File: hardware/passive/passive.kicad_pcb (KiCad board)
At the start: 2 copper layers, 45 x 17 mm, 8 parts, among them J1 i/O, J2 Conn 1, J3 Conn 2

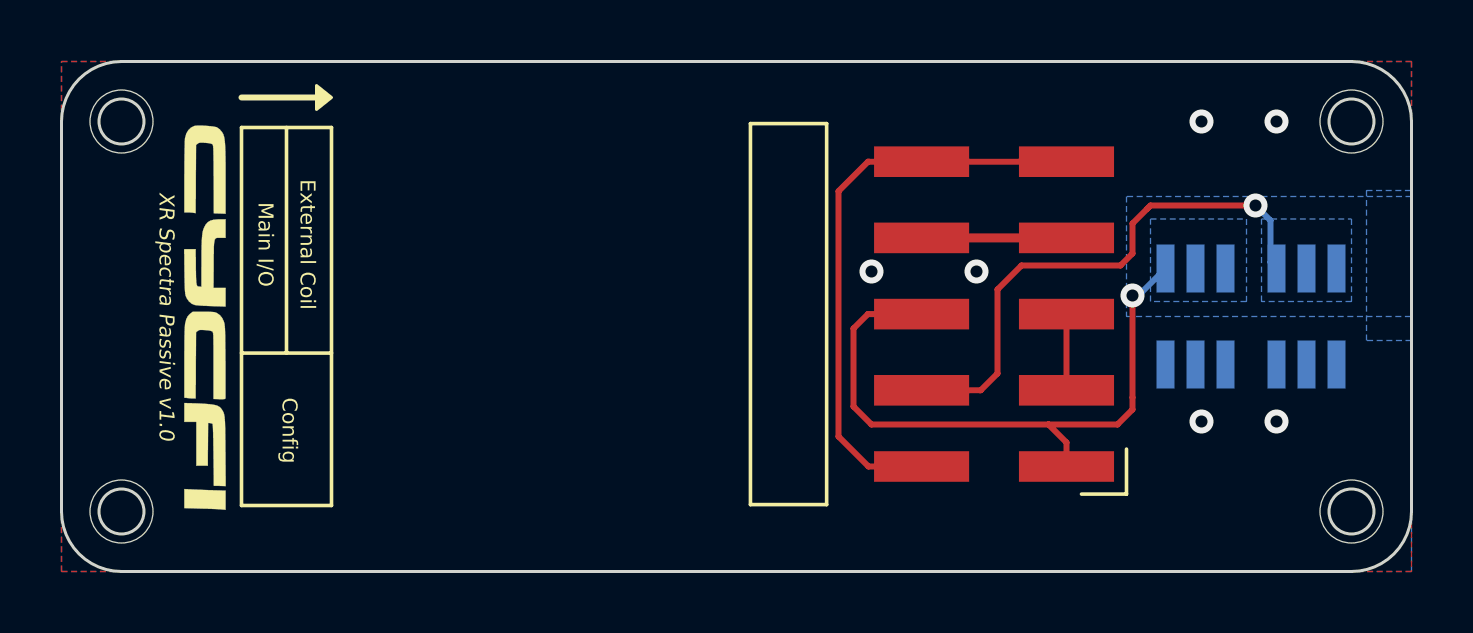
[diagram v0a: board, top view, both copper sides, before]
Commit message: Passive board updates
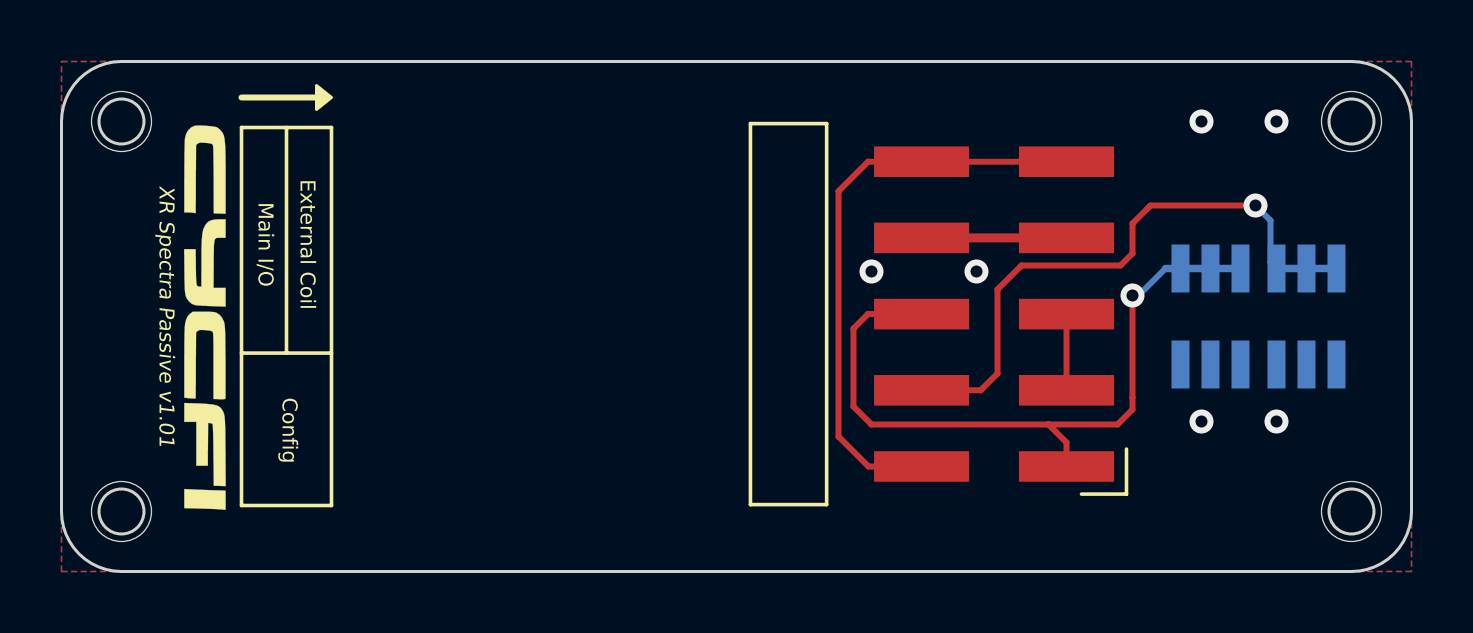
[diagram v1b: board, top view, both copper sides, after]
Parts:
- H1, H2, H3, H4: footprint cycfi_library:mounting_hole_2.1mm -> cycfi_library:mounting_hole_st1.9; moved to F.Cu
- moved J3 0.50 mm to (143.3, 108.5)
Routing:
- net out-: track 21.7 -> 24.2 mm
- net int_coil+: track 18.3 -> 20.3 mm
- removed copper zone on B.Cu, net int_coil+
- removed copper zone on B.Cu, net out-
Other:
- board text added: "XR Spectra Passive v1.01"
- board text removed: "XR Spectra Passive v1.0"
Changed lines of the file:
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@@
     (thickness 1.6)
     (drawings 24)
-    (tracks 42)
+    (tracks 47)
     (zones 0)
     (modules 8)
@@
     (44 Edge.Cuts user)
     (45 Margin user)
-    (46 B.CrtYd user hide)
-    (47 F.CrtYd user hide)
-    (48 B.Fab user hide)
-    (49 F.Fab user hide)
+    (46 B.CrtYd user)
+    (47 F.CrtYd user)
+    (48 B.Fab user)
+    (49 F.Fab user)
   )
   (setup
@@
     (add_net out-)
   )
+  (module cycfi_library:mounting_hole_st1.9 (layer F.Cu)
+    (at 148 115)
+    (descr "Mounting Hole 2.1mm, no annular")
+    (tags "mounting hole 2.1mm no annular")
+    (attr virtual)
+    (fp_text reference H4 (at 0 -3.2) (layer F.SilkS) hide
+      (effects (font (size 1 1) (thickness 0.15)))
+    )
+    (fp_text value MountingHole (at 0 3.2) (layer F.Fab) hide
+      (effects (font (size 1 1) (thickness 0.15)))
+    )
+    (fp_text user %R (at 0.3 0) (layer F.Fab)
+      (effects (font (size 1 1) (thickness 0.15)))
+    )
+    (fp_circle (center 0 0) (end 1.75 0) (layer F.CrtYd) (width 0.05))
+    (pad "" np_thru_hole circle (at 0 0) (size 2 2) (drill 2) (layers *.Cu *.Mask))
+  )
+  (module cycfi_library:mounting_hole_st1.9 (layer F.Cu)
+    (at 148 102)
+    (descr "Mounting Hole 2.1mm, no annular")
+    (tags "mounting hole 2.1mm no annular")
+    (attr virtual)
+    (fp_text reference H3 (at 0 -3.2 180) (layer F.SilkS) hide
+      (effects (font (size 1 1) (thickness 0.15)))
+    )
+    (fp_text value MountingHole (at 0 3.2 180) (layer F.Fab) hide
+      (effects (font (size 1 1) (thickness 0.15)))
+    )
+    (fp_text user %R (at 0.3 0 180) (layer F.Fab)
+      (effects (font (size 1 1) (thickness 0.15)))
+    )
+    (fp_circle (center 0 0) (end 1.75 0) (layer F.CrtYd) (width 0.05))
+    (pad "" np_thru_hole circle (at 0 0) (size 2 2) (drill 2) (layers *.Cu *.Mask))
+  )
+  (module cycfi_library:mounting_hole_st1.9 (layer F.Cu)
+    (at 107 115)
+    (descr "Mounting Hole 2.1mm, no annular")
+    (tags "mounting hole 2.1mm no annular")
+    (attr virtual)
+    (fp_text reference H2 (at 0 -3.2) (layer F.SilkS) hide
+      (effects (font (size 1 1) (thickness 0.15)))
+    )
+    (fp_text value MountingHole (at 0 3.2) (layer F.Fab) hide
+      (effects (font (size 1 1) (thickness 0.15)))
+    )
+    (fp_text user %R (at 0.3 0) (layer F.Fab)
+      (effects (font (size 1 1) (thickness 0.15)))
+    )
+    (fp_circle (center 0 0) (end 1.75 0) (layer F.CrtYd) (width 0.05))
+    (pad "" np_thru_hole circle (at 0 0) (size 2 2) (drill 2) (layers *.Cu *.Mask))
+  )
+  (module cycfi_library:mounting_hole_st1.9 (layer F.Cu)
+    (at 107 102)
+    (descr "Mounting Hole 2.1mm, no annular")
+    (tags "mounting hole 2.1mm no annular")
+    (attr virtual)
+    (fp_text reference H1 (at 0 -3.2) (layer F.SilkS) hide
+      (effects (font (size 1 1) (thickness 0.15)))
+    )
+    (fp_text value MountingHole (at 0 3.2) (layer F.Fab) hide
+      (effects (font (size 1 1) (thickness 0.15)))
+    )
+    (fp_text user %R (at 0.3 0) (layer F.Fab)
+      (effects (font (size 1 1) (thickness 0.15)))
+    )
+    (fp_circle (center 0 0) (end 1.75 0) (layer F.CrtYd) (width 0.05))
+    (pad "" np_thru_hole circle (at 0 0) (size 2 2) (drill 2) (layers *.Cu *.Mask))
+  )
   (module cycfi_library:pin_socket_2x3p_1.00mm_smd_vertical (layer B.Cu)
     (at 146.5 108.5 90)
@@
   )
   (module cycfi_library:pin_socket_2x3p_1.00mm_smd_vertical (layer B.Cu)
-    (at 142.8 108.5 90)
+    (at 143.3 108.5 90)
     (descr "surface-mounted straight pin header, 2x03, 1.00mm pitch, double rows")
     (tags "Surface mounted pin header SMD 2x03 1.00mm double row")
@@
       (rotate (xyz 0 0 0))
     )
-  )
-  (module cycfi_library:mounting_hole_2.1mm (layer B.Cu)
-    (at 148 115)
-    (descr "Mounting Hole 2.1mm, no annular")
-    (tags "mounting hole 2.1mm no annular")
-    (attr virtual)
-    (fp_text reference H4 (at 0 3.2) (layer B.SilkS) hide
-      (effects (font (size 1 1) (thickness 0.15)) (justify mirror))
-    )
-    (fp_text value MountingHole (at 0 -3.2) (layer B.Fab)
-      (effects (font (size 1 1) (thickness 0.15)) (justify mirror))
-    )
-    (fp_text user %R (at 0.3 0) (layer B.Fab)
-      (effects (font (size 1 1) (thickness 0.15)) (justify mirror))
-    )
-    (fp_circle (center 0 0) (end 2.35 0) (layer B.CrtYd) (width 0.05))
-    (pad "" np_thru_hole circle (at 0 0) (size 2.1 2.1) (drill 2.1) (layers *.Cu *.Mask))
-  )
-  (module cycfi_library:mounting_hole_2.1mm (layer B.Cu)
-    (at 148 102)
-    (descr "Mounting Hole 2.1mm, no annular")
-    (tags "mounting hole 2.1mm no annular")
-    (attr virtual)
-    (fp_text reference H3 (at 0 3.2) (layer B.SilkS) hide
-      (effects (font (size 1 1) (thickness 0.15)) (justify mirror))
-    )
-    (fp_text value MountingHole (at 0 -3.2) (layer B.Fab)
-      (effects (font (size 1 1) (thickness 0.15)) (justify mirror))
-    )
-    (fp_text user %R (at 0.3 0) (layer B.Fab)
-      (effects (font (size 1 1) (thickness 0.15)) (justify mirror))
-    )
-    (fp_circle (center 0 0) (end 2.35 0) (layer B.CrtYd) (width 0.05))
-    (pad "" np_thru_hole circle (at 0 0) (size 2.1 2.1) (drill 2.1) (layers *.Cu *.Mask))
-  )
-  (module cycfi_library:mounting_hole_2.1mm (layer B.Cu)
-    (at 107 115)
-    (descr "Mounting Hole 2.1mm, no annular")
-    (tags "mounting hole 2.1mm no annular")
-    (attr virtual)
-    (fp_text reference H2 (at 0 3.2) (layer B.SilkS) hide
-      (effects (font (size 1 1) (thickness 0.15)) (justify mirror))
-    )
-    (fp_text value MountingHole (at 0 -3.2) (layer B.Fab)
-      (effects (font (size 1 1) (thickness 0.15)) (justify mirror))
-    )
-    (fp_text user %R (at 0.3 0) (layer B.Fab)
-      (effects (font (size 1 1) (thickness 0.15)) (justify mirror))
-    )
-    (fp_circle (center 0 0) (end 2.35 0) (layer B.CrtYd) (width 0.05))
-    (pad "" np_thru_hole circle (at 0 0) (size 2.1 2.1) (drill 2.1) (layers *.Cu *.Mask))
-  )
-  (module cycfi_library:mounting_hole_2.1mm (layer B.Cu)
-    (at 107 102)
-    (descr "Mounting Hole 2.1mm, no annular")
-    (tags "mounting hole 2.1mm no annular")
-    (attr virtual)
-    (fp_text reference H1 (at 0 3.2) (layer B.SilkS) hide
-      (effects (font (size 1 1) (thickness 0.15)) (justify mirror))
-    )
-    (fp_text value MountingHole (at 0 -3.2) (layer B.Fab)
-      (effects (font (size 1 1) (thickness 0.15)) (justify mirror))
-    )
-    (fp_text user %R (at 0.3 0) (layer B.Fab)
-      (effects (font (size 1 1) (thickness 0.15)) (justify mirror))
-    )
-    (fp_circle (center 0 0) (end 2.35 0) (layer B.CrtYd) (width 0.05))
-    (pad "" np_thru_hole circle (at 0 0) (size 2.1 2.1) (drill 2.1) (layers *.Cu *.Mask))
   )
   (module cycfi_library:cycfi-logo-12mm (layer F.Cu)
@@
   (gr_line (start 114 114.8) (end 111 114.8) (layer F.SilkS) (width 0.12))
   (gr_line (start 114 102.2) (end 114 114.8) (layer F.SilkS) (width 0.12))
-  (gr_text "XR Spectra Passive v1.0" (at 108.5 108.5 -90) (layer F.SilkS)
+  (gr_text "XR Spectra Passive v1.01" (at 108.5 108.5 -90) (layer F.SilkS)
     (effects (font (size 0.5 0.5) (thickness 0.125) italic))
   )
@@
   (segment (start 145.3 106.7) (end 145.5 106.9) (width 0.2) (layer B.Cu) (net 4))
   (segment (start 145.3 105.3) (end 145.3 106.7) (width 0.2) (layer B.Cu) (net 4))
+  (segment (start 145.5 106.9) (end 146.5 106.9) (width 0.25) (layer B.Cu) (net 4))
+  (segment (start 146.5 106.9) (end 147.5 106.9) (width 0.25) (layer B.Cu) (net 4))
   (segment (start 138.5 112.7) (end 138.5 113.5) (width 0.2) (layer F.Cu) (net 5))
   (segment (start 137.9 112.1) (end 138.5 112.7) (width 0.2) (layer F.Cu) (net 5))
@@
   (segment (start 140.7 111.6) (end 140.7 111.2) (width 0.2) (layer F.Cu) (net 5))
   (segment (start 140.2 112.1) (end 140.7 111.6) (width 0.2) (layer F.Cu) (net 5))
+  (segment (start 141.8 106.9) (end 142.3 106.9) (width 0.25) (layer B.Cu) (net 5))
+  (segment (start 142.3 106.9) (end 143.3 106.9) (width 0.25) (layer B.Cu) (net 5))
+  (segment (start 143.3 106.9) (end 144.3 106.9) (width 0.25) (layer B.Cu) (net 5))
   (zone (net 1) (net_name GND) (layer F.Cu) (hatch edge 0.508)
-    (connect_pads yes (clearance 0.254))
+    (connect_pads (clearance 0.254))
     (min_thickness 0.254)
     (fill yes (arc_segments 32) (thermal_gap 0.508) (thermal_bridge_width 0.508))
@@
     )
   )
-  (zone (net 4) (net_name int_coil+) (layer B.Cu) (hatch edge 0.508)
-    (connect_pads yes (clearance 0.254))
+  (zone (net 1) (net_name GND) (layer B.Cu) (hatch edge 0.508)
+    (connect_pads (clearance 0.254))
     (min_thickness 0.254)
     (fill yes (arc_segments 32) (thermal_gap 0.508) (thermal_bridge_width 0.508))
     (polygon
       (pts
-        (xy 148 108) (xy 145 108) (xy 145 105.25) (xy 148 105.25)
+        (xy 150 117) (xy 105 117) (xy 105 100) (xy 150 100)
       )
     )
-  )
-  (zone (net 1) (net_name GND) (layer B.Cu) (hatch edge 0.508)
-    (connect_pads yes (clearance 0.254))
-    (min_thickness 0.254)
-    (fill yes (arc_segments 32) (thermal_gap 0.508) (thermal_bridge_width 0.508))
-    (polygon
-      (pts
-        (xy 150 109.3) (xy 148.5 109.3) (xy 148.5 104.3) (xy 150 104.3)
-      )
-    )
-  )
-  (zone (net 1) (net_name GND) (layer B.Cu) (hatch edge 0.508)
-    (connect_pads yes (clearance 0.254))
-    (min_thickness 0.254)
-    (fill yes (arc_segments 32) (thermal_gap 0.508) (thermal_bridge_width 0.508))
-    (polygon
-      (pts
-        (xy 150 104.5) (xy 140.5 104.5) (xy 140.5 108.5) (xy 150 108.5) (xy 150 117)
-        (xy 105 117) (xy 105 100) (xy 150 100)
-      )
-    )
-  )
-  (zone (net 5) (net_name out-) (layer B.Cu) (hatch edge 0.508)
-    (connect_pads yes (clearance 0.2))
-    (min_thickness 0.2)
-    (fill yes (arc_segments 32) (thermal_gap 0.5) (thermal_bridge_width 0.5))
-    (polygon
-      (pts
-        (xy 144.5 108) (xy 141.3 108) (xy 141.3 105.25) (xy 144.5 105.25)
-      )
-    )

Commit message: updates for v1.01
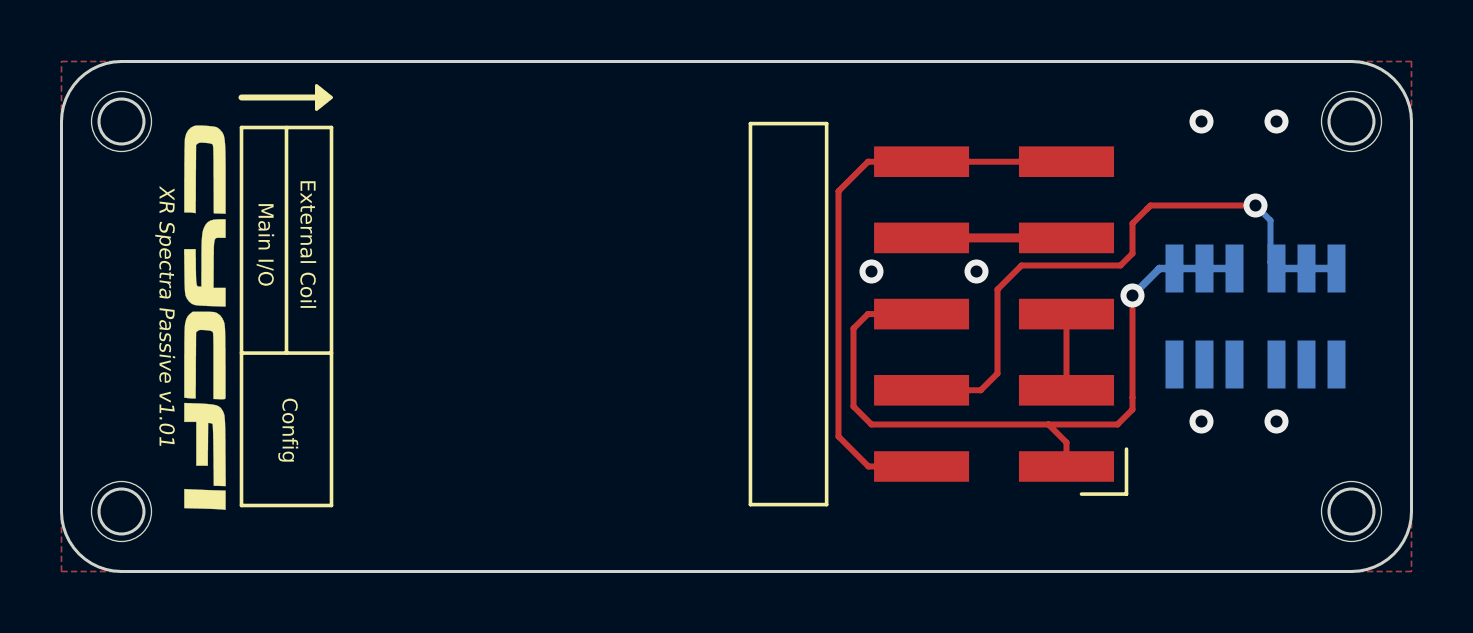
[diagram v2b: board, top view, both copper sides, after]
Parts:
- moved J3 0.20 mm to (143.1, 108.5)
